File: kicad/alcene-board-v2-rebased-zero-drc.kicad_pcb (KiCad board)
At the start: 2 copper layers, 109.3 x 87.1 mm, 16 parts, among them J1 ESP32-S3-DevKitC-1_J1, J2 USB-C Input, J3 ESP32-S3-DevKitC-1_J3, J4 ILI9341_TFT_14pin, J5 Male Pin Header 1x18 - J1 Sig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, J6 Male Pin Header 1x18 - J3 Sig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, J7 Male Pin Header 2x4 - GND, J8 Male Pin Header 2x4 - 3V3, J9 Male Pin Header 2x4 - VIN 5V, SW1 ESP32-S3 Reset (NO momentary)

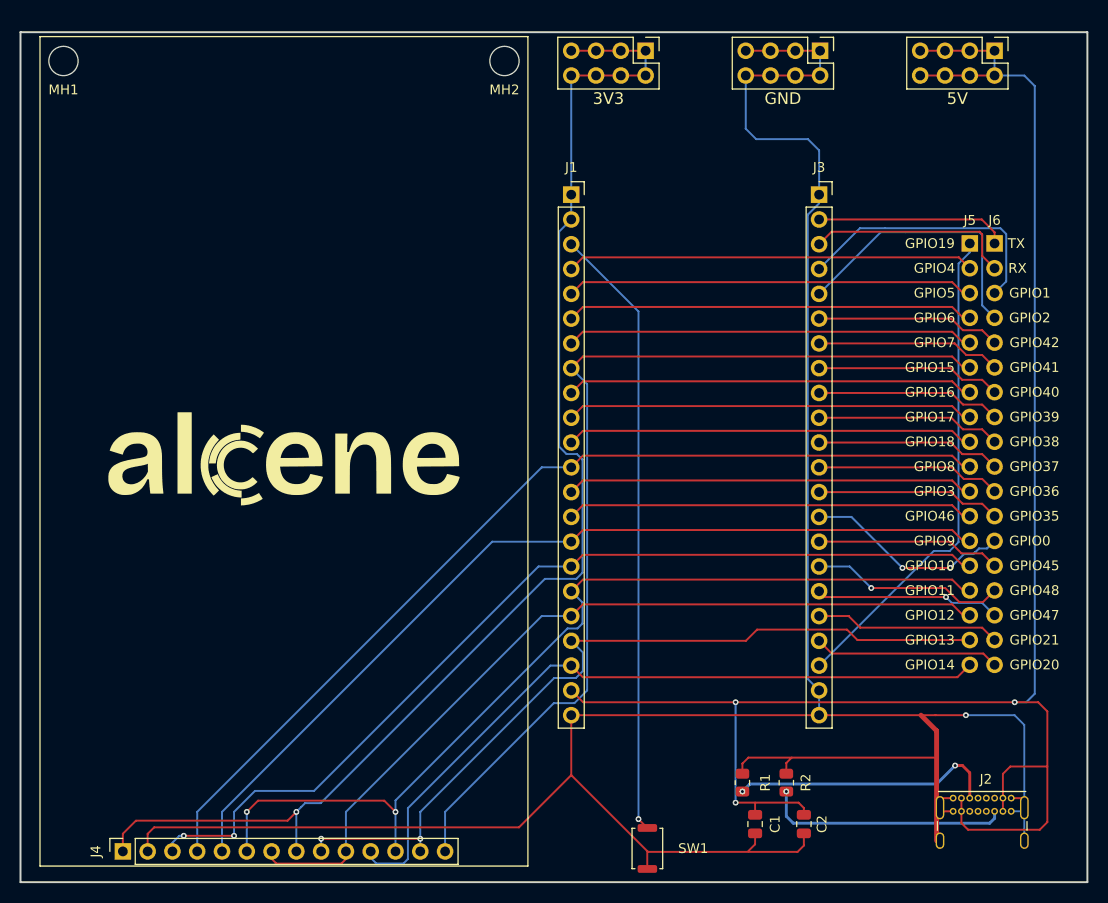
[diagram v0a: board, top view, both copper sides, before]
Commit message: feat: final layout r2
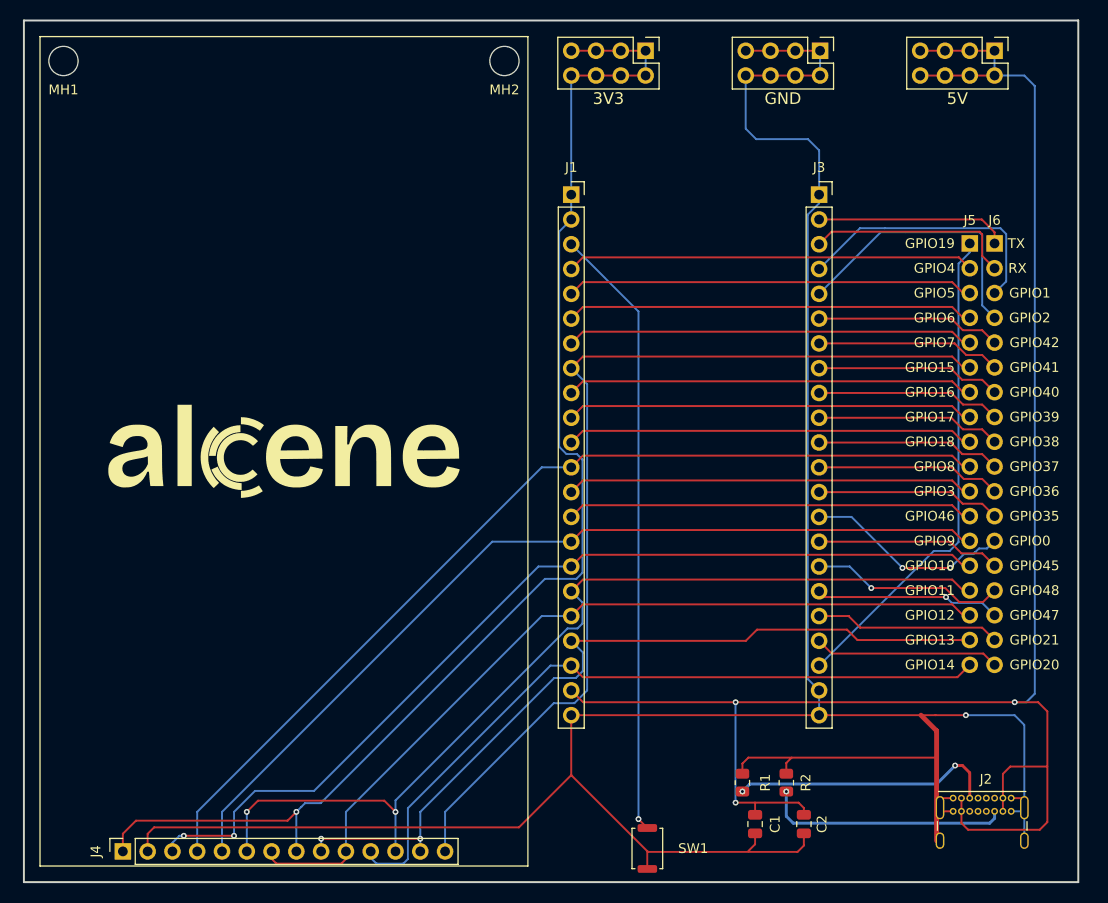
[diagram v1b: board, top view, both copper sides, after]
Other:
- board size 109.3 x 87.1 mm -> 108 x 88.3 mm
